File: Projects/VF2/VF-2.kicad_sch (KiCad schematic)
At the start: 23 parts, among them Q1 MPSA42, Q2 MPSA92, Q3 IRF540N, Q4 IRF9540N, U1 Opa2134, U4 OPA2134

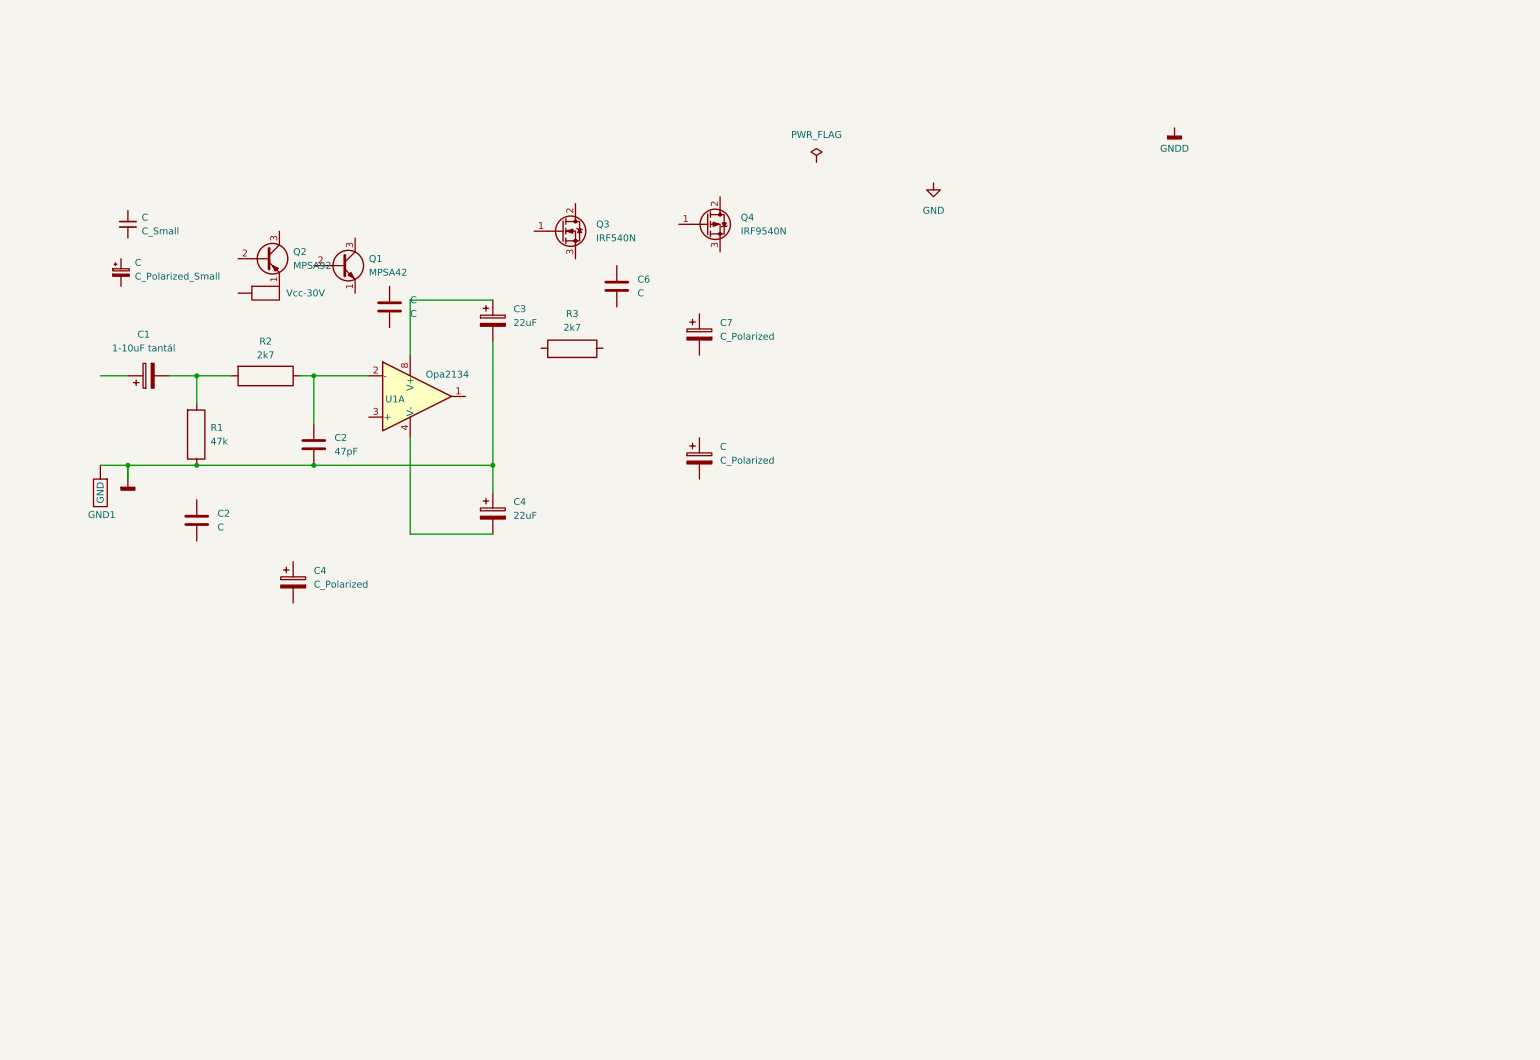
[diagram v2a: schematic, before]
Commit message: sch
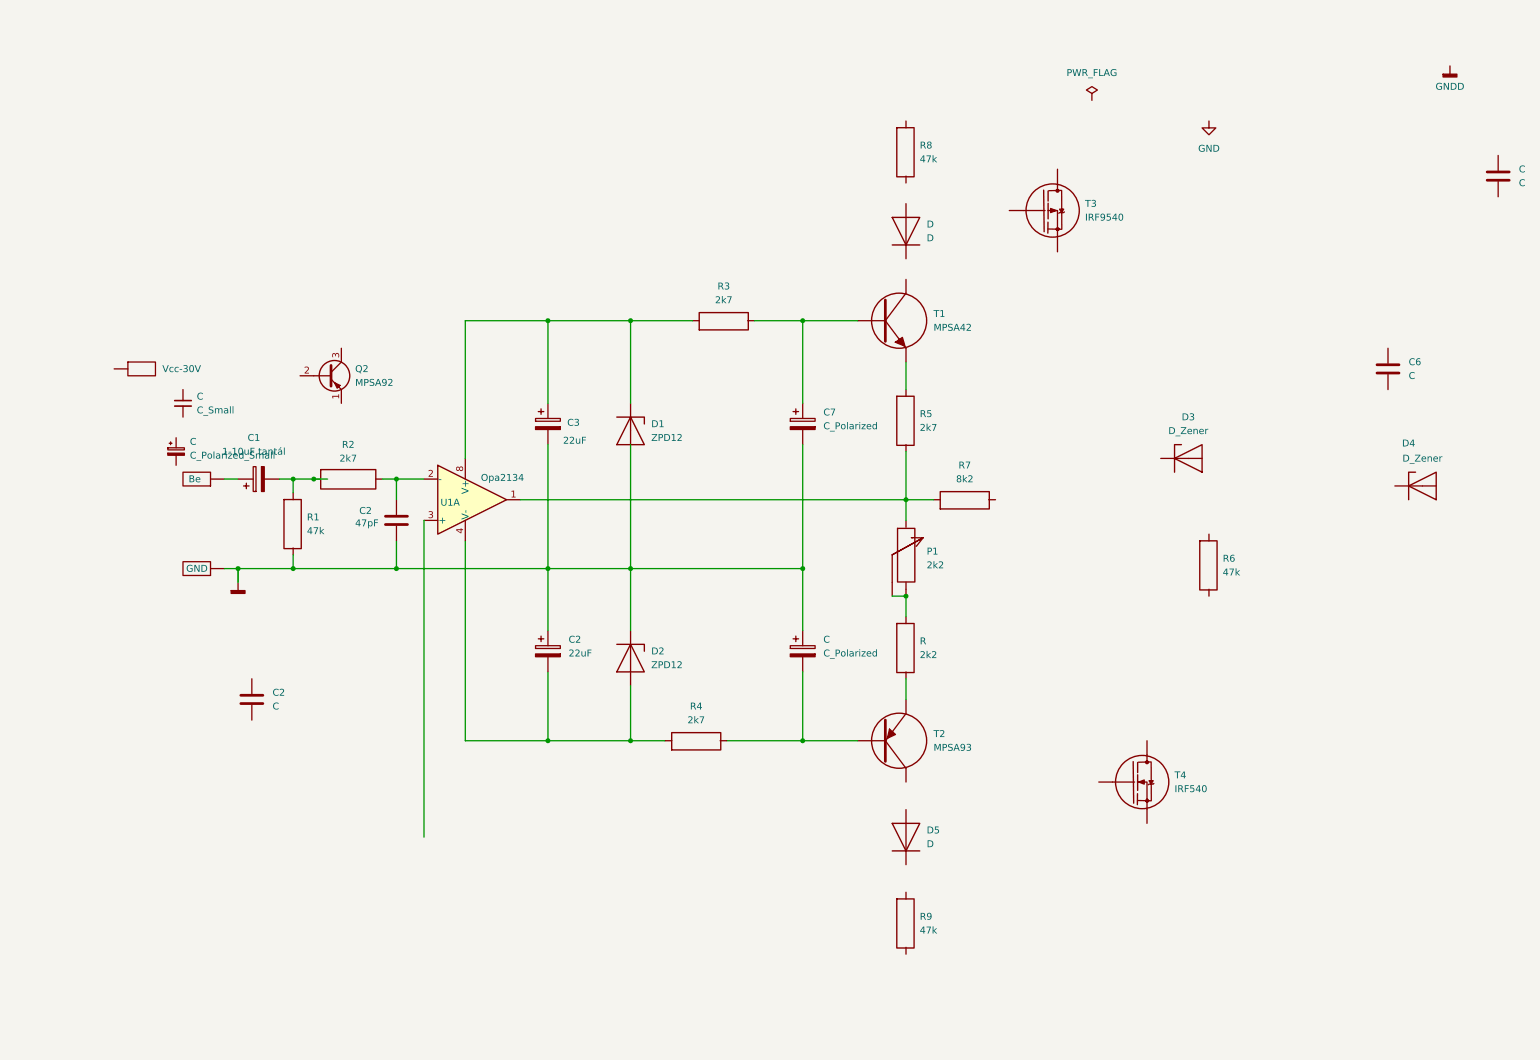
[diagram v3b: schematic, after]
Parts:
- removed C4: 22uF, Package_SO:SOIC-8_3.9x4.9mm_P1.27mm, symbol 001_Capacitor_user:C_Polarized
- removed Q1: MPSA42, Package_TO_SOT_THT:TO-92_Inline, symbol Transistor_BJT:MPSA42
- removed Q3: IRF540N, Package_TO_SOT_THT:TO-220-3_Vertical, symbol Transistor_FET:IRF540N
- added Be: (no value), Diode_SMD:Littelfuse_PolyZen-LS, symbol 001_atmeneti_Device:Vcc
- added D, D5: D, Diode_THT:D_DO-35_SOD27_P7.62mm_Horizontal, symbol Diode:1N4148
- added D1: ZPD12, Diode_SMD:Littelfuse_PolyZen-LS, symbol Device:D_Zener
- added D2: ZPD12, Diode_SMD:Littelfuse_PolyZen-LS, symbol 000_Device:D_Zener
- added D3, D4: D_Zener, Diode_SMD:Littelfuse_PolyZen-LS, symbol 000_Device:D_Zener
- added P1: 2k2, Diode_THT:D_DO-35_SOD27_P7.62mm_Horizontal, symbol Device:R_Trim
- added R: 2k2, symbol 001_Resistor_user:R_álló
- added R4: 2k7, Package_SO:SOIC-8_3.9x4.9mm_P1.27mm, symbol 000_Device:R
- added R5: 2k7, symbol 001_Resistor_user:R_álló
- added R6, R8, R9: 47k, symbol 001_Resistor_user:R_álló
- added R7: 8k2, symbol 001_Resistor_user:R_álló
- added T1: MPSA42, Package_TO_SOT_THT:TO-92_Inline, symbol 000_Device:NPN_Transistor
- added T2: MPSA93, Package_TO_SOT_THT:TO-92_Inline, symbol 000_Device:PNP_Transistor
- added T4: IRF540, Package_TO_SOT_THT:TO-220-3_Vertical, symbol 000_Device:N_Channel_FET
- C2: renamed from C4; value C_Polarized -> 22uF
- T3: renamed from Q4; value IRF9540N -> IRF9540
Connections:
- net at C.1: now also C2.1, C2.2, C3.2, C7.2, GND1. (GND), R1.1, D1.2 (A), D2.1 (K)
- net at C.2: now also R4.1, T2. (E)
- net at U4.4 (V-): now also C2.2, D2.2 (A), R4.2
- net at C3.1, U4.8 (V+): now also R3.2, D1.1 (K)
- net at C7.1: now also R3.1, T1. (E)
- net at C1.1: now also Be.
- net at U1.1: now also P1.1, R5.1, R7.2
- new net: P1., P1.2, R.2
- new net: R5.2, T1. (E)
- new net: R.1, T2. (E)
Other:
- moved on the sheet: C, C1, C2, C3, C6, C7, Q2, R1, R2, R3, U1A, Vcc-30V

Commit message: sch
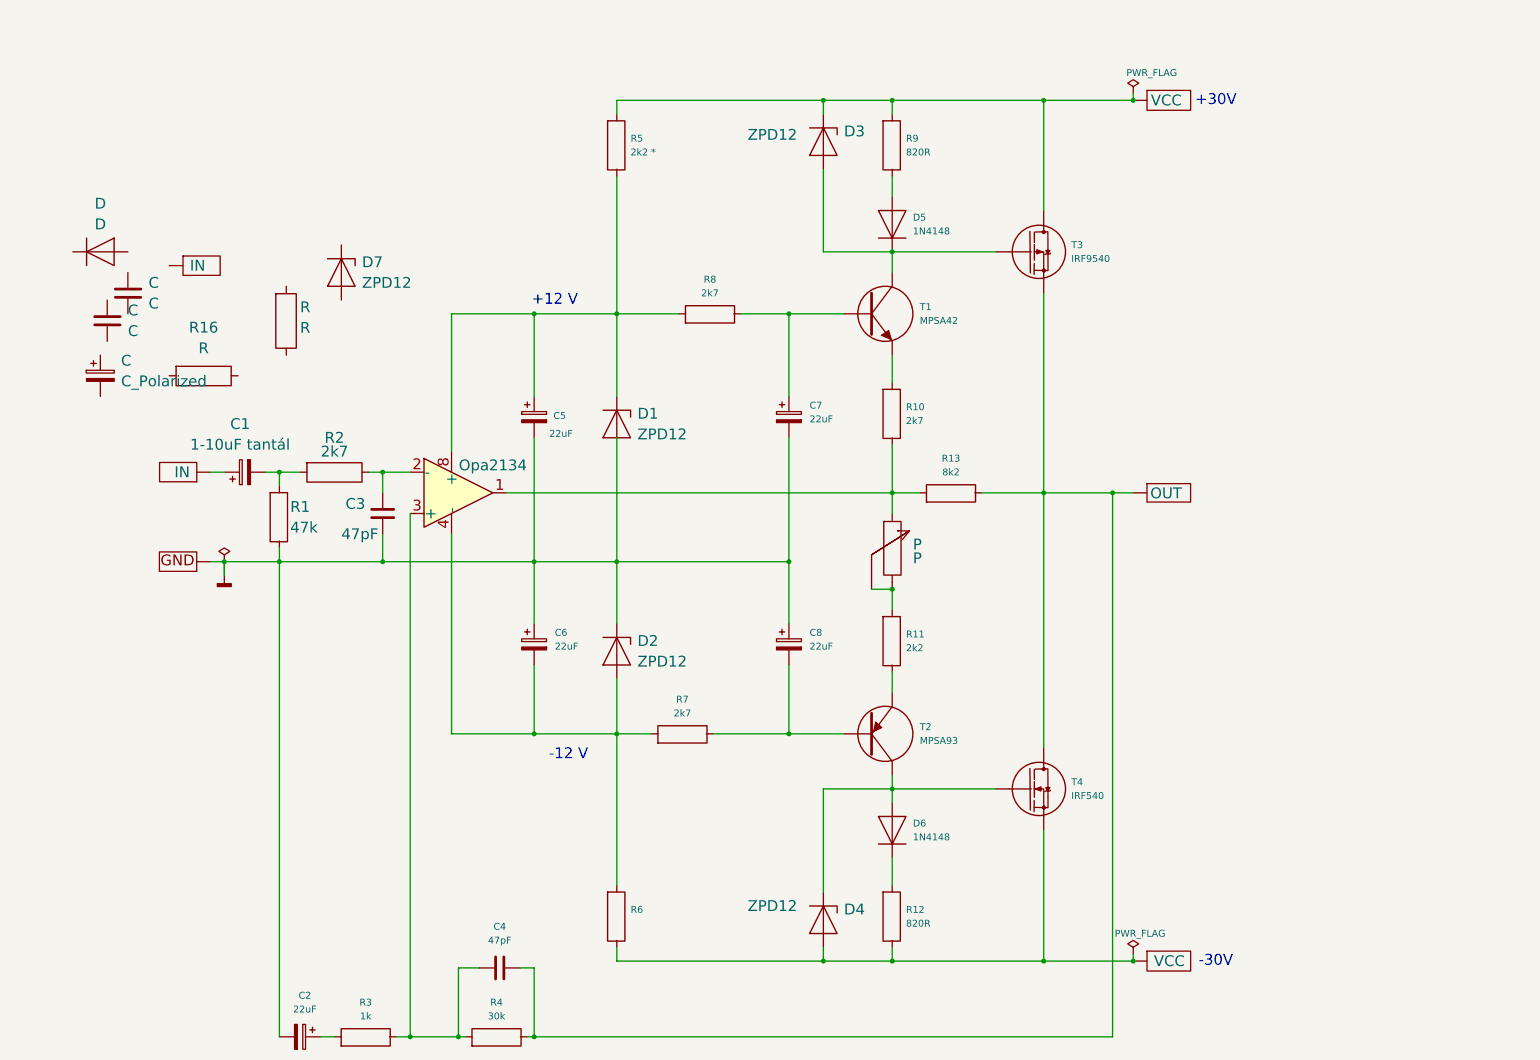
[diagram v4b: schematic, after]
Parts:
- removed C: C_Polarized_Small, Package_SO:SOIC-8_3.9x4.9mm_P1.27mm, symbol Device:C_Polarized_Small
- removed C: C_Small, symbol Device:C_Small
- removed C: C, Package_SO:SOIC-8_3.9x4.9mm_P1.27mm, symbol 001_Capacitor_user:C
- removed C2, C6: C, Package_SO:SOIC-8_3.9x4.9mm_P1.27mm, symbol 000_Device:C
- removed Q2: MPSA92, Package_TO_SOT_THT:TO-92_Inline, symbol Transistor_BJT:MPSA92
- removed R6: 47k, symbol 001_Resistor_user:R_álló
- added C: C, Package_SO:SOIC-8_3.9x4.9mm_P1.27mm, symbol 000_Device:C
- added C: C_Polarized, Package_SO:SOIC-8_3.9x4.9mm_P1.27mm, symbol 000_Device:C_Polarized
- added C: C, Package_SO:SOIC-8_3.9x4.9mm_P1.27mm, symbol 000_Device:C_Polarized
- added C2: 22uF, Package_SO:SOIC-8_3.9x4.9mm_P1.27mm, symbol 000_Device:C_Polarized
- added C4: 47pF, Package_SO:SOIC-8_3.9x4.9mm_P1.27mm, symbol 001_atmeneti_user_library:C
- added D: D, Diode_THT:D_DO-35_SOD27_P7.62mm_Horizontal, symbol 000_Device:D
- added D7: ZPD12, Diode_SMD:Littelfuse_PolyZen-LS, symbol 000_Device:D_Zener
- added IN: (no value), Diode_SMD:Littelfuse_PolyZen-LS, symbol 000_Device:Bemenet
- added OUT: (no value), Diode_SMD:Littelfuse_PolyZen-LS, symbol 000_Device:Kimenet
- added R: R, symbol 000_Device:R_álló
- added R16: R, symbol 000_Device:R
- added R3: 1k, Package_SO:SOIC-8_3.9x4.9mm_P1.27mm, symbol 000_Device:R
- added R4: 30k, Package_SO:SOIC-8_3.9x4.9mm_P1.27mm, symbol 000_Device:R
- added R5: 2k2 *, symbol 000_Device:R
- added R6: 2k2*, symbol 000_Device:R
- added Vcc2: VCC, Diode_THT:D_DO-35_SOD27_P7.62mm_Horizontal, symbol 000_Device:Vcc
- C7: value C_Polarized -> 22uF
- C8: renamed from C; value C_Polarized -> 22uF
- D3, D4: value D_Zener -> ZPD12
- D5: renamed from D; value D -> 1N4148
- D6: renamed from D5; value D -> 1N4148
- P: renamed from P1; value 2k2 -> P
- R12: renamed from R9; value 47k -> 820R
- R9: renamed from R8; value 47k -> 820R
- Vcc1: renamed from Vcc-30V; value (none) -> VCC
- renumbered C2 to C3, C3 to C5, C2 to C6, Be to IN, R5 to R10, R to R11, R7 to R13, R4 to R7, R3 to R8, U4 to U2
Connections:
- net GND: now also C3.2, C5.2, C6.1, C7.2, C8.1, D1.2 (A), D2.1 (K), GND1., R1.1, C2.2
- net at Vcc1.: now also D3.1 (K), R9.2, T3. (S), R5.2
- net at T4. (S): now also D4.1 (K), D6.2 (A), T2. (E)
- net at D5.1 (K): now also D3.2 (A), T1. (E), T3. (S)
- net at D5.2 (A): now also R9.1
- net at C5.1, D1.1 (K), R8.2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: now also R5.1
- net at T1. (E): now also R10.2
- net at C6.2, D2.2 (A), R7.2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: now also R6.2
- net at R13.1: now also T3. (S), T4. (S), C4.2, OUT., R4.1
- net at D4.2 (A): now also R12.1, T4. (S), R6.1, Vcc2.
- net at R12.2: now also D6.1 (K)
- net at U1.3 (+): now also C4.1, R3.1, R4.2
- new net: C2.1, R3.2
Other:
- note added: "+12 V"
- note added: "+30V"
- note added: "-12 V"
- note added: "-30V"
- moved on the sheet: C1, C3, C5, C6, C7, C8, D1, D2, D5, D6, IN, P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
